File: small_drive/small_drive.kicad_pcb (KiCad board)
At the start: 2 copper layers, 100 x 80 mm, 159 parts, among them J1 DB9, J2 DB15, M1 SiR826DP, M2 SiR826DP, M3 SiR826DP, M4 SiR826DP, M5 SiR826DP, M6 SiR826DP, P1 CONN_01X04, P2 CONN_01X04, P3 CONN_01X04, P4 CONN_01X04, P5 CONN_01X02, P6 CONN_01X02, P7 CONN_01X02, P8 CONN_01X01, U1 XMC4400-F64x512, U10 LM5106, U11 ACS711KLCTR-12AB-T, U12 ACS711ELCTR-25AB-T, U13 ACS711KLCTR-12AB-T, U14 AD8226, U15 MAX3096, U16 AMC1203, U17 7805, U18 LT1764EQ, U19 KSZ8081, U2 ips511g, U20 ETH100_MAG, U3 ips511g, U4 LTC2850, U5 AD8226, U6 LT1764EQ, U7 MC33074DTBR2, U8 LM5106, U9 LM5106, X1 NKE1212DC, X2 NKE1212DC, X3 HCPL0201, X4 HCPL0201, X5 HCPL0201, X6 HCPL0201, Y1 12MHz, Y2 25MHz

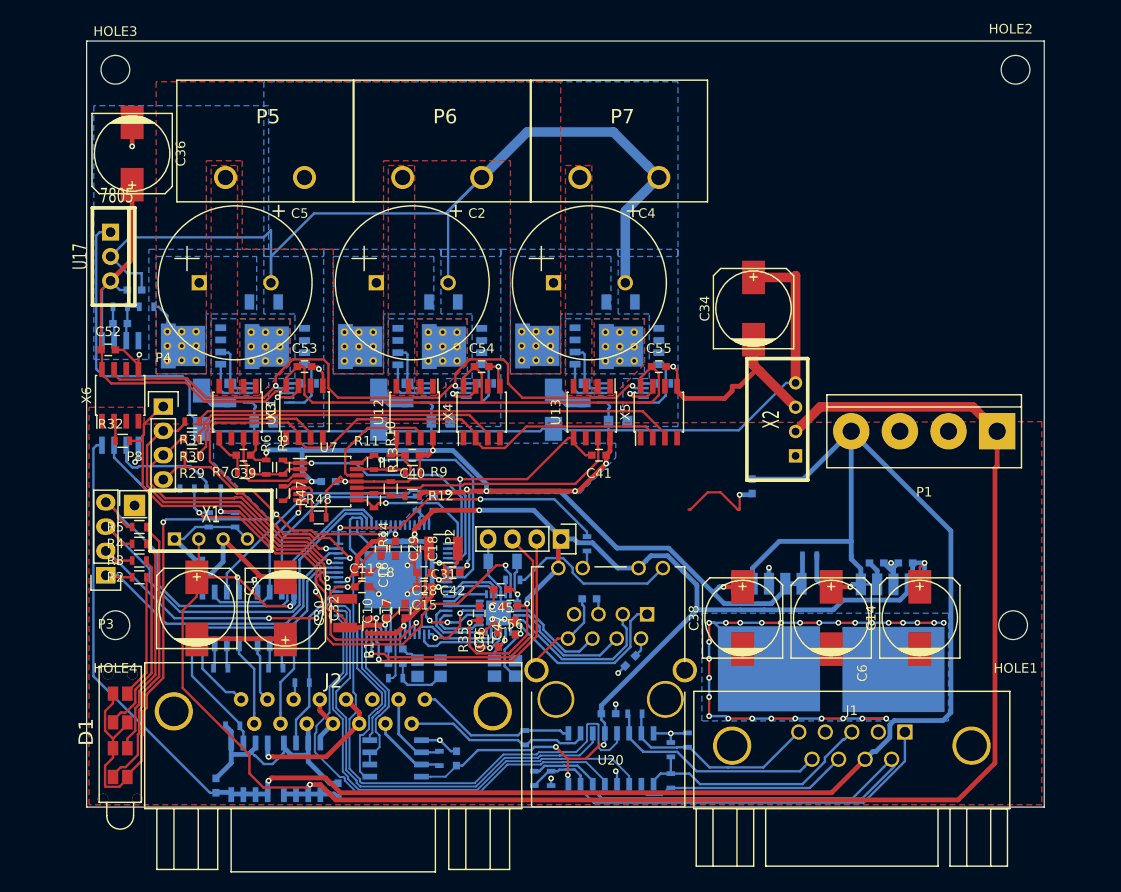
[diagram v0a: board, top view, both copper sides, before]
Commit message: PCB ordered.
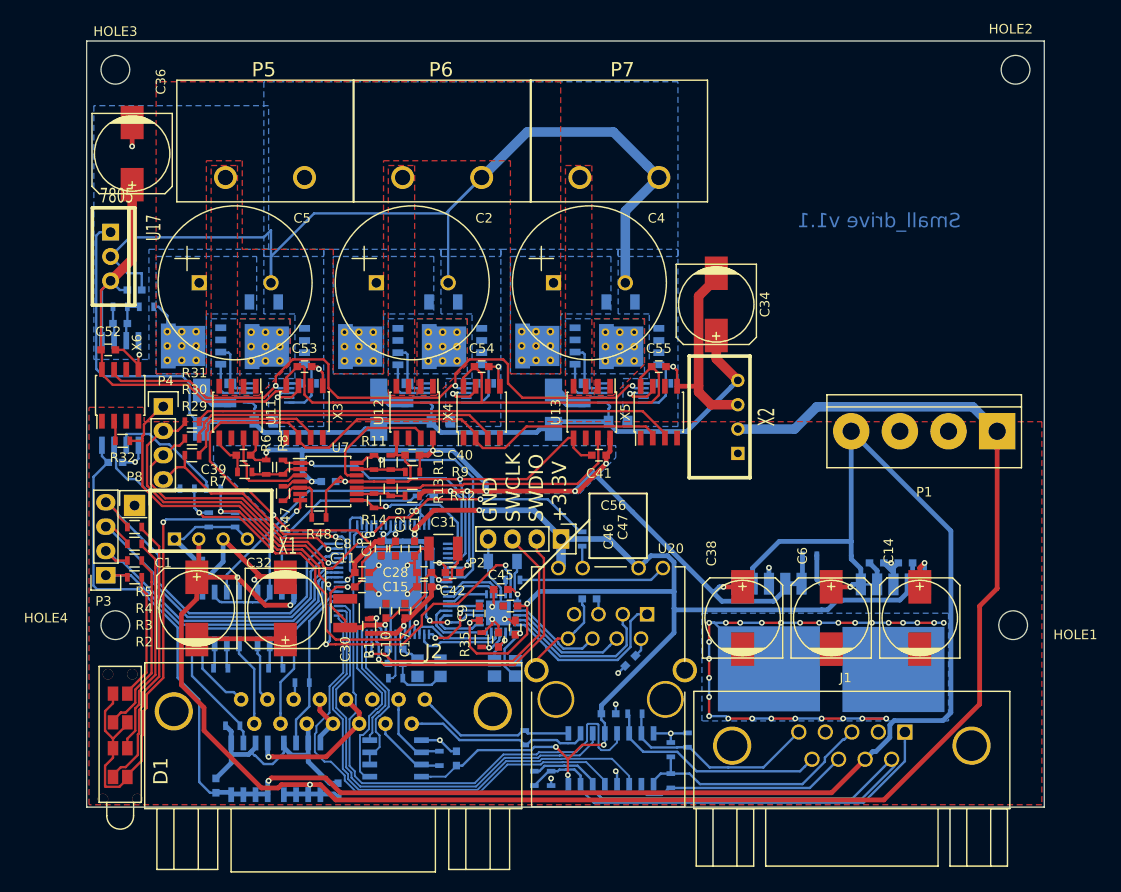
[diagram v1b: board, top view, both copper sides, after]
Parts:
- moved C13 66.5 mm to (42.0, 148.0), turned to 0 degrees
- moved X2 6.04 mm to (107.0, 143.2)
- moved C34 3.91 mm to (104.8, 131.5), turned to 270 degrees
- moved R37 0.71 mm to (90.8, 156.0)
- moved R2 0.50 mm to (44.0, 160.0)
- moved R3 0.50 mm to (44.0, 158.2)
- moved R4 0.50 mm to (44.0, 156.5)
- moved R5 0.50 mm to (44.0, 154.8)
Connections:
- net Net-(P2-Pad2) renamed /SWDIO
- net Net-(P2-Pad3) renamed /SWCLK
- U1 pad 3: /LED2 -> /HBEN
- U1 pad 4: /LED3 -> /LED4
- U1 pad 52: /LED1 -> /ETH0_~RST
- U1 pad 57: /HBEN -> /ENC_5V
- U1 pad 58: /ETH0_~RST -> /LED0
- U1 pad 59: /ENC_5V -> /LED1
- U1 pad 62: /LED0 -> /LED2
- U1 pad 64: /LED4 -> /LED3
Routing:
- net +12P: track 122.3 -> 105.8 mm
- net +5V: track 211.8 -> 202.3 mm
- net +3.3V: track 317.4 -> 326.7 mm
- net GND: track 272.0 -> 263.9 mm, vias 48 -> 47
- net +3.3VADC: track 125.9 -> 117.9 mm
- net /LED2: track 43.2 -> 36.5 mm
- net Net-(J2-Pad2): track 15.1 -> 8.72 mm
- net Net-(J2-Pad10): track 14.2 -> 8.08 mm
- net /LED3: track 45.7 -> 39.6 mm
- net /LED4: track 30.7 -> 25.8 mm
- net /HBEN: track 35.8 -> 40.2 mm
- net /ETH0_~RST: track 35.5 -> 31.4 mm
- net Net-(R36-Pad1): track 17.9 -> 15.4 mm
- net /LED1: track 31.4 -> 33.7 mm, vias 2 -> 0
- net Net-(R25-Pad2): track 11.8 -> 10.2 mm
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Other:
- board text added: "GND SWCLK SWDIO +3.3V"
- board text added: "Small_drive v1.1"
- board text removed: "+"
